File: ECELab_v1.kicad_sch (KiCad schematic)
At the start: 0 parts

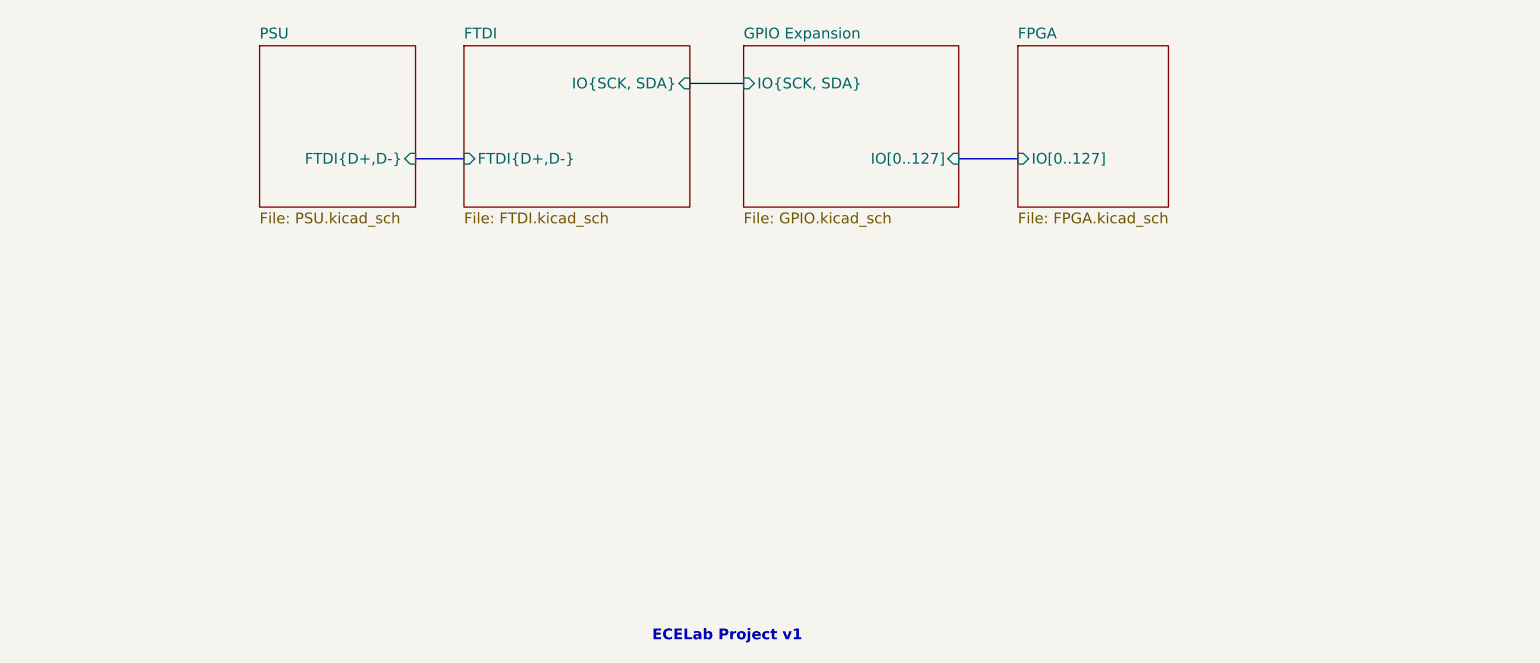
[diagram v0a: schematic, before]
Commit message: Complete Draft 1 of PCB Design
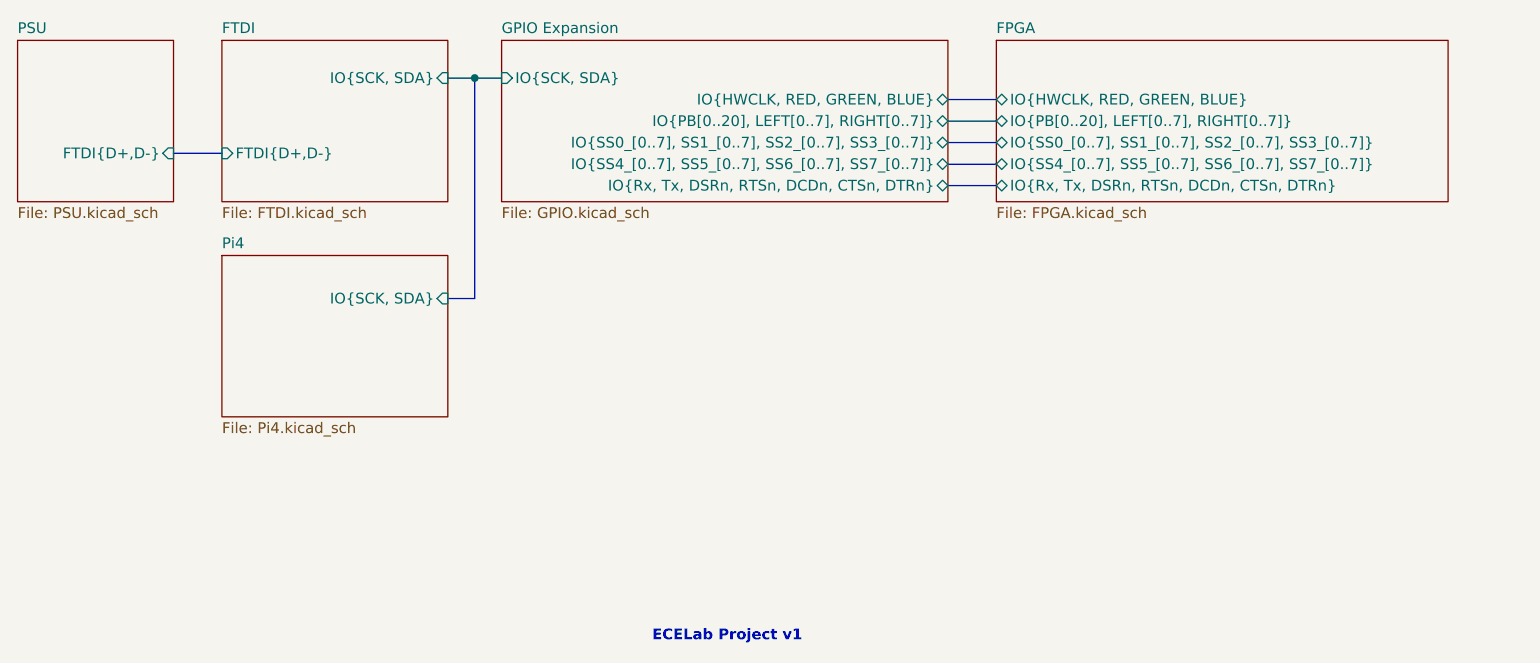
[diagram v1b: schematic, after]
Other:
- added sheet Pi4 (Pi4.kicad_sch)
- sheet FPGA ports: added IO{HWCLK, RED, GREEN, BLUE}, IO{PB[0..20], LEFT[0..7], RIGHT[0..7]}, IO{Rx, Tx, DSRn, RTSn, DCDn, CTSn, DTRn}, IO{SS0_[0..7], SS1_[0..7], SS2_[0..7], SS3_[0..7]}, IO{SS4_[0..7], SS5_[0..7], SS6_[0..7], SS7_[0..7]}; removed IO[0..127]
- sheet GPIO Expansion ports: added IO{HWCLK, RED, GREEN, BLUE}, IO{PB[0..20], LEFT[0..7], RIGHT[0..7]}, IO{Rx, Tx, DSRn, RTSn, DCDn, CTSn, DTRn}, IO{SS0_[0..7], SS1_[0..7], SS2_[0..7], SS3_[0..7]}, IO{SS4_[0..7], SS5_[0..7], SS6_[0..7], SS7_[0..7]}; removed IO[0..127]
